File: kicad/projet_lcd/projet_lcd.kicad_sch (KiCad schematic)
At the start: 0 parts

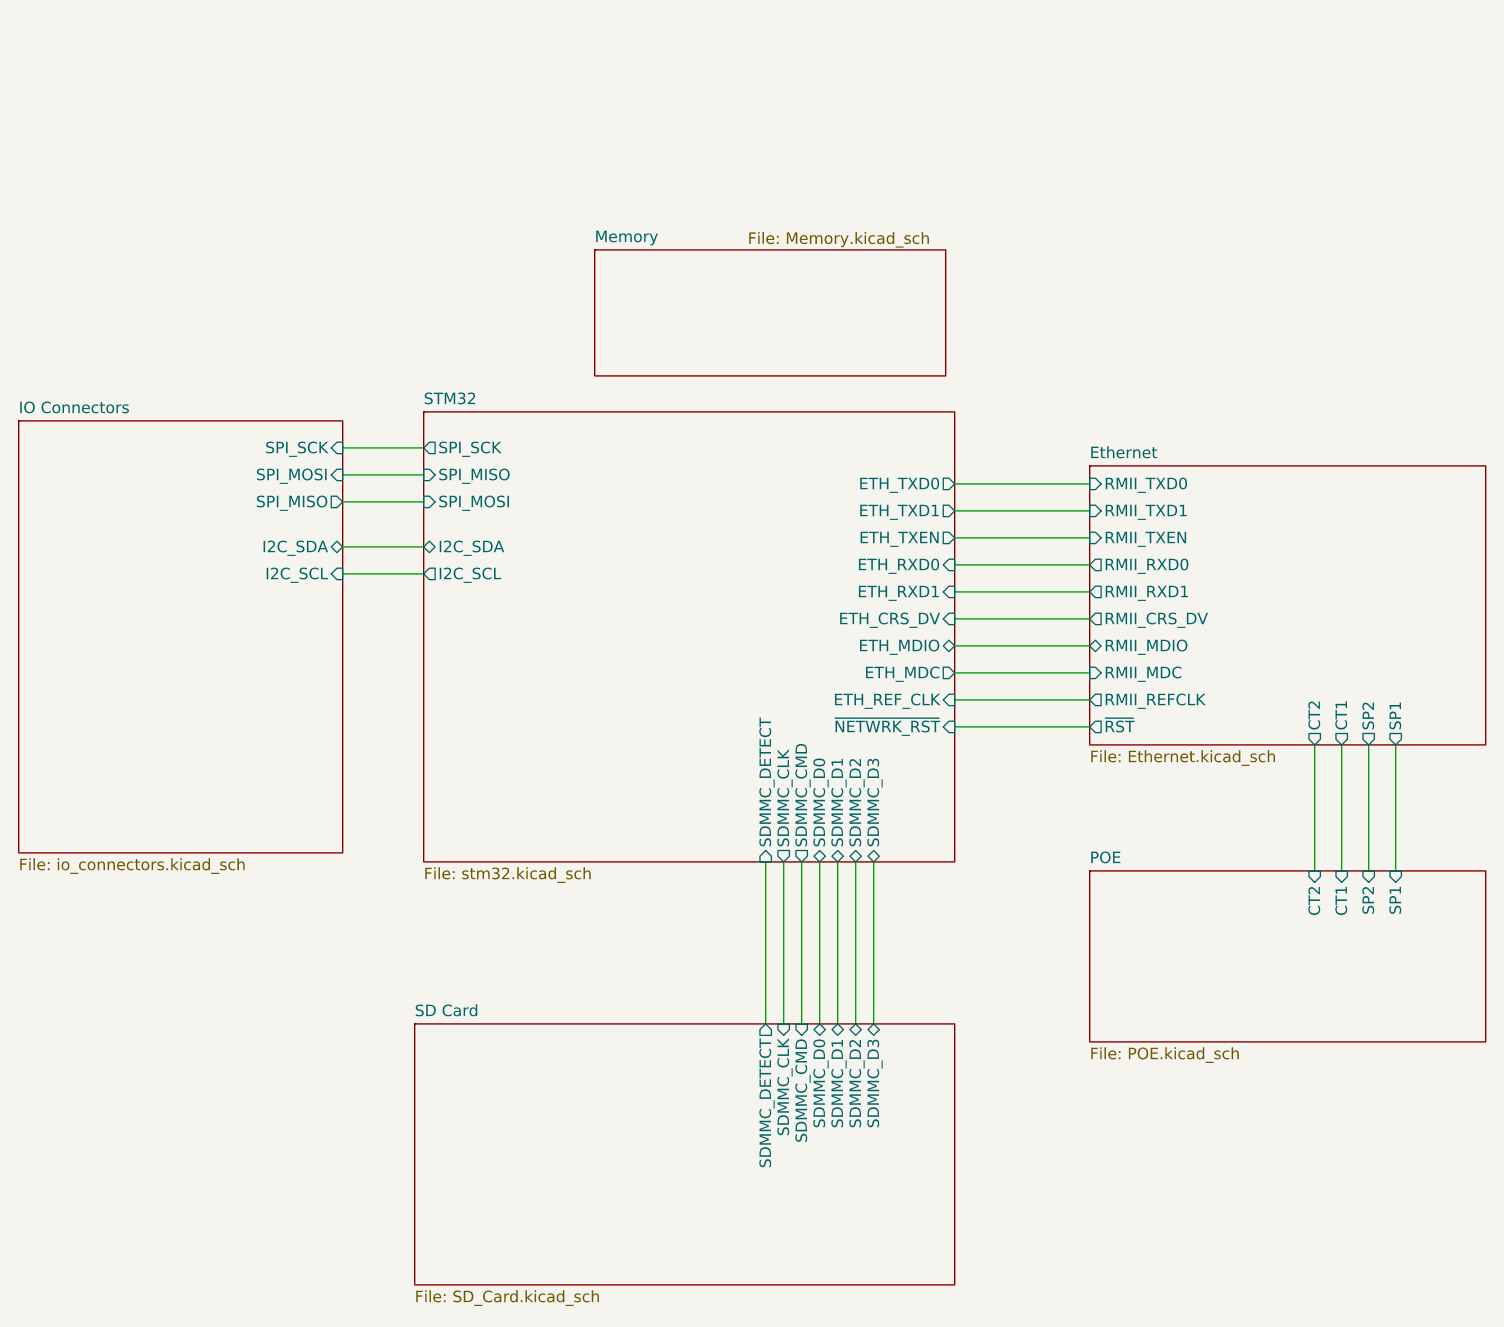
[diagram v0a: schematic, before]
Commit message: on avance !
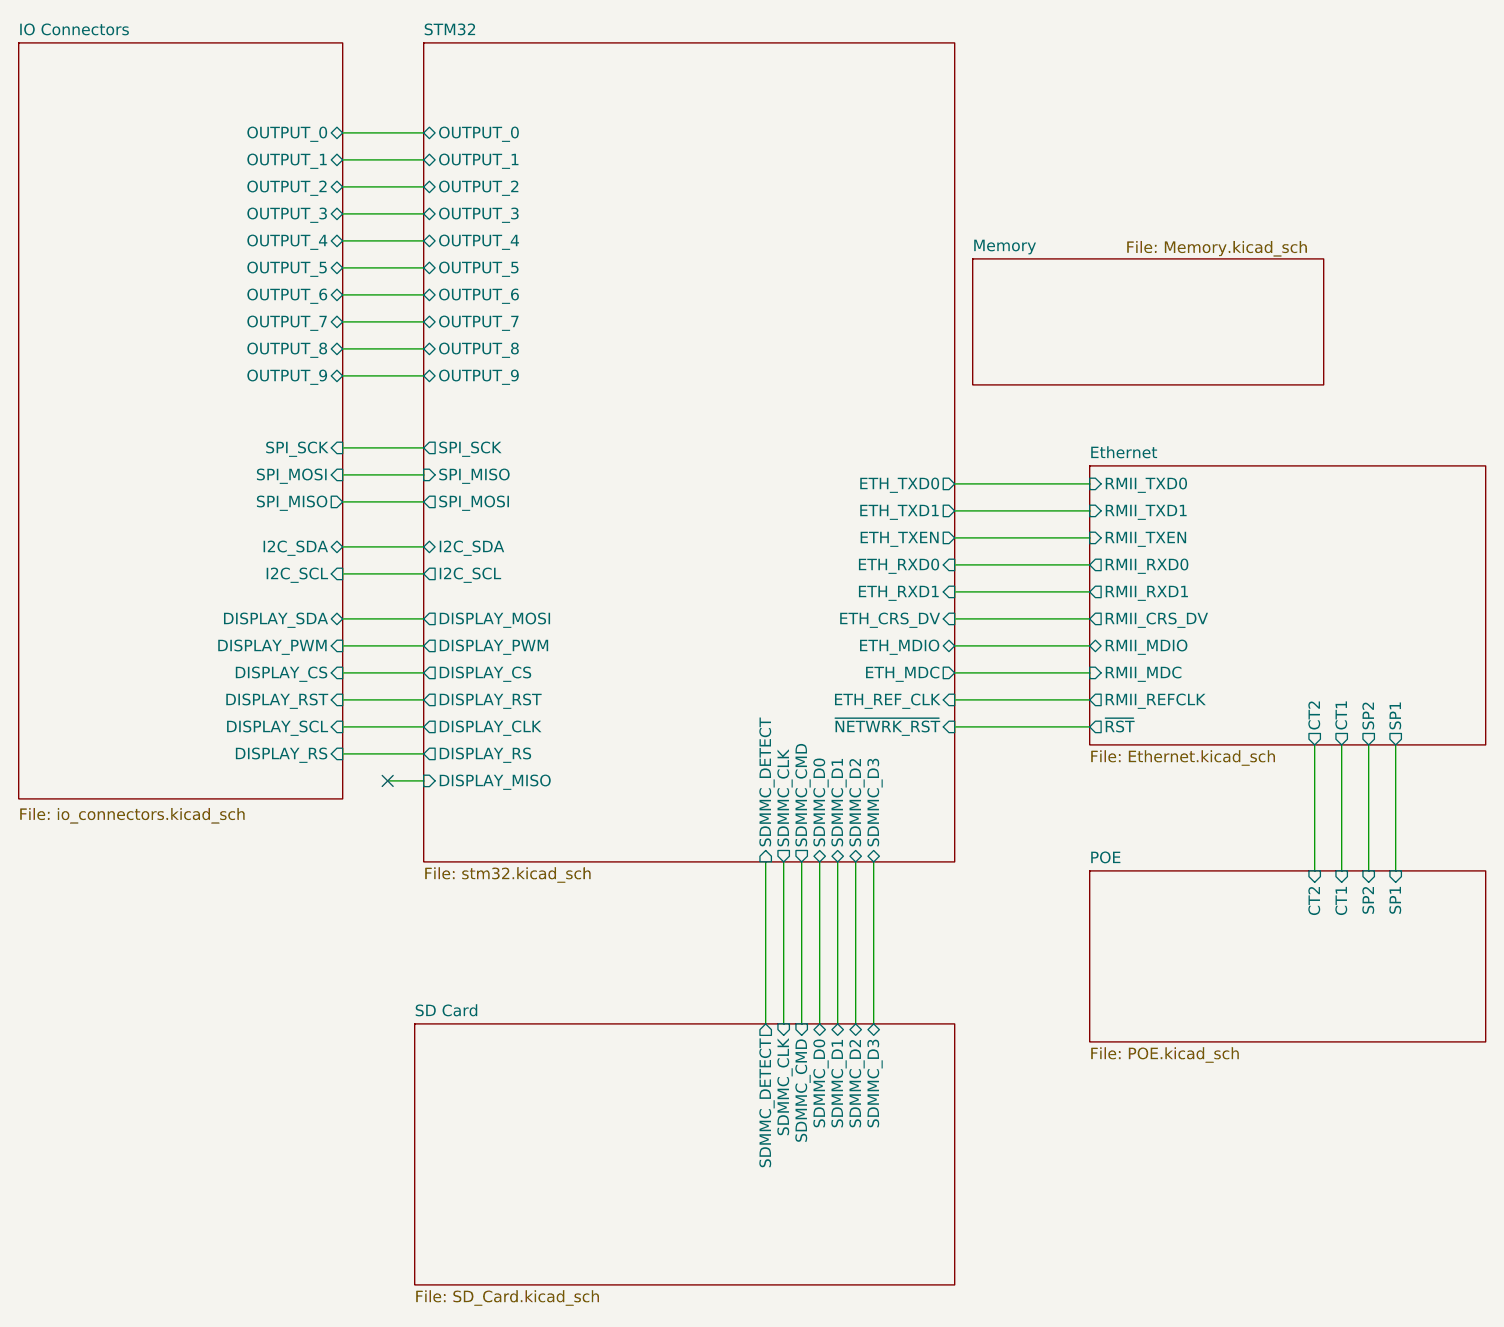
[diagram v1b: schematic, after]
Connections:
- no-connect marks 0 -> 1
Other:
- sheet IO Connectors ports: added DISPLAY_CS, DISPLAY_PWM, DISPLAY_RS, DISPLAY_RST, DISPLAY_SCL, DISPLAY_SDA, OUTPUT_0, OUTPUT_1, OUTPUT_2, OUTPUT_3, OUTPUT_4, OUTPUT_5, OUTPUT_6, OUTPUT_7, OUTPUT_8, OUTPUT_9; removed none
- sheet STM32 ports: added DISPLAY_CLK, DISPLAY_CS, DISPLAY_MISO, DISPLAY_MOSI, DISPLAY_PWM, DISPLAY_RS, DISPLAY_RST, OUTPUT_0, OUTPUT_1, OUTPUT_2, OUTPUT_3, OUTPUT_4, OUTPUT_5, OUTPUT_6, OUTPUT_7, OUTPUT_8, OUTPUT_9; removed none
